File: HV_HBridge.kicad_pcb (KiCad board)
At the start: 2 copper layers, 1 part

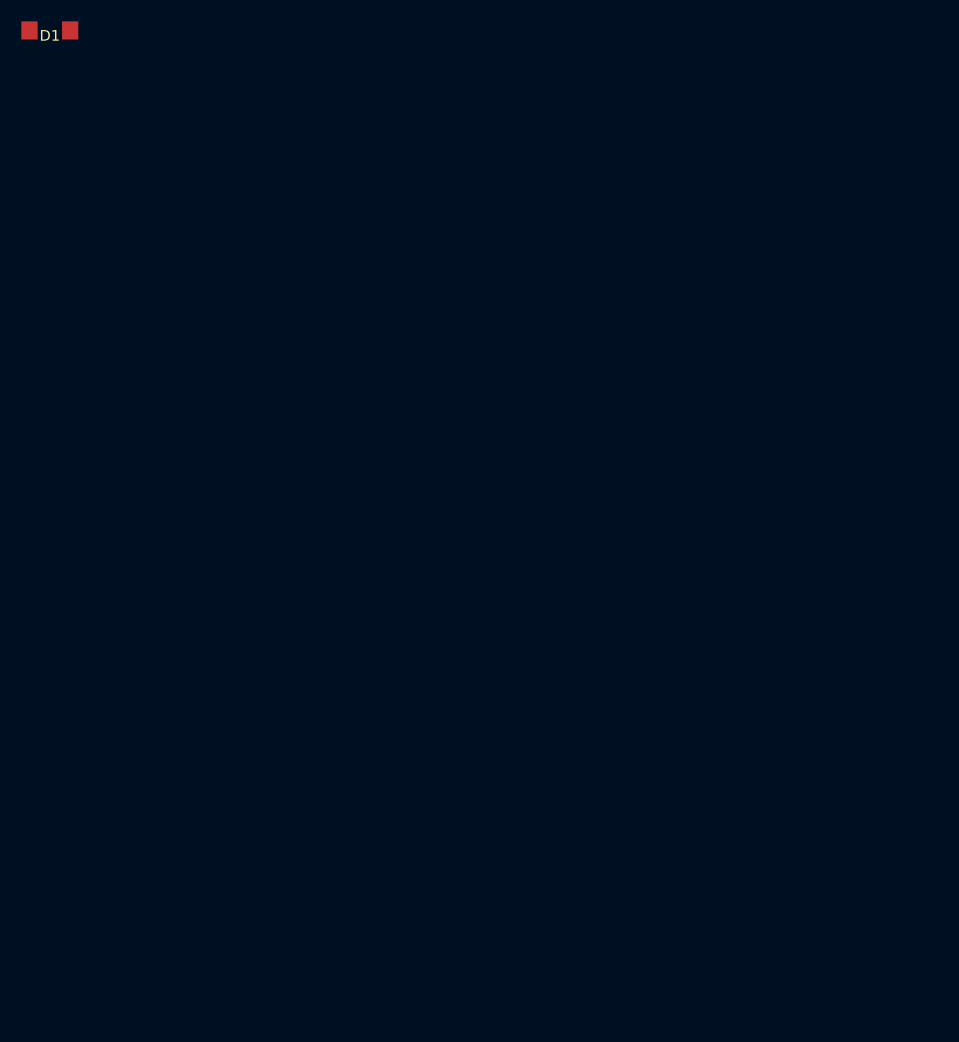
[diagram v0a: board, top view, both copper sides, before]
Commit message: updated to latest version
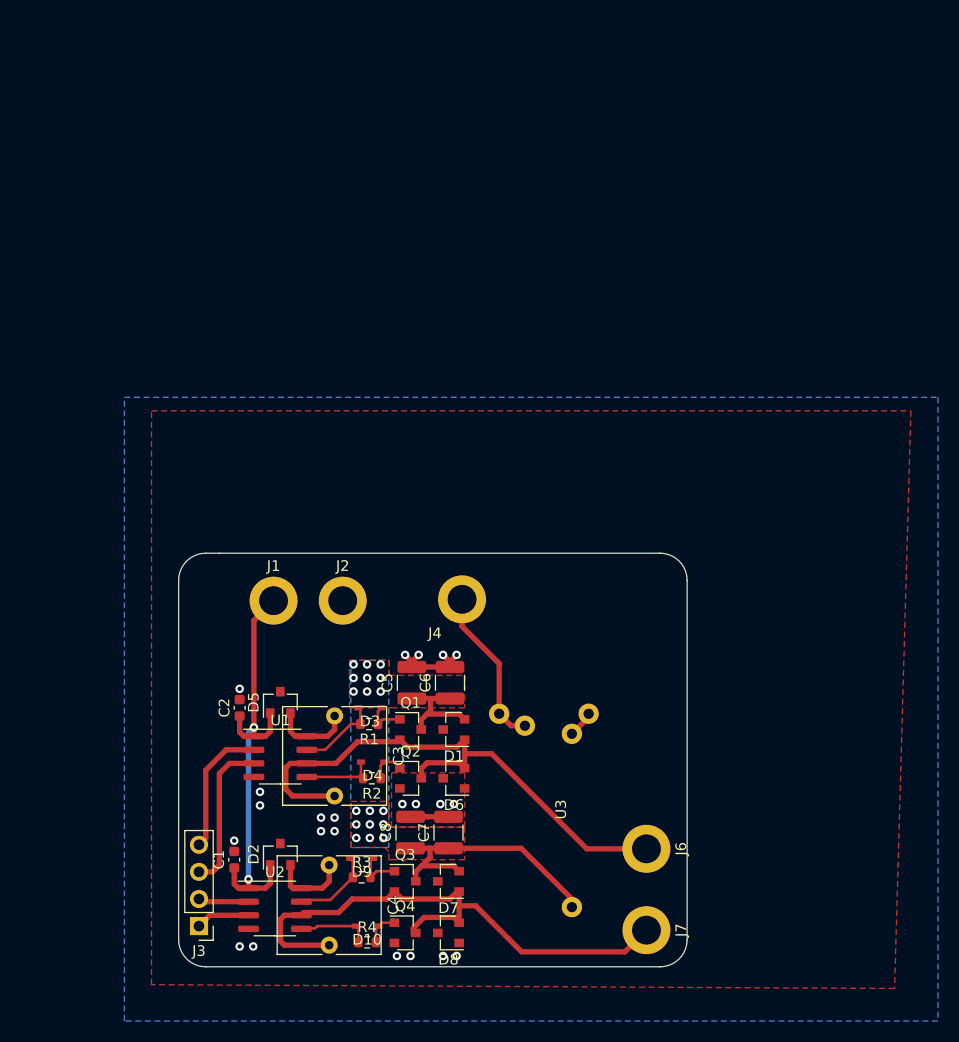
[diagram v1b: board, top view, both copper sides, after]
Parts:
- added C1: 100n 25V, Capacitor_SMD:C_0603_1608Metric, F.Cu at (106.8, 68.7)
- added C2: 100n 25V, Capacitor_SMD:C_0603_1608Metric, F.Cu at (107.3, 54.5)
- added C3: 1u 630V, Capacitor_THT:C_Rect_L9.0mm_W9.5mm_P7.50mm_MKT, F.Cu at (116.2, 55.2)
- added C4: 1u 630V, Capacitor_THT:C_Rect_L9.0mm_W9.5mm_P7.50mm_MKT, F.Cu at (115.7, 69.2)
- added C5: 100n 630V, Capacitor_SMD:C_1210_3225Metric, F.Cu at (123.4, 52.1)
- added C6: 100n 630V, Capacitor_SMD:C_1210_3225Metric, F.Cu at (127.0, 52.1)
- added C7: 100n 630V, Capacitor_SMD:C_1210_3225Metric, F.Cu at (126.9, 66.2)
- added C8: 100n 630V, Capacitor_SMD:C_1210_3225Metric, F.Cu at (123.3, 66.2)
- added D10: D, HBREMS_Hbridge:SOD-323, F.Cu at (119.3, 74.9)
- added D2: BAS101, Package_TO_SOT_SMD:SOT-23, F.Cu at (111.1, 68.2)
- added D3: D, HBREMS_Hbridge:SOD-323, F.Cu at (119.5, 54.5)
- added D4: D, HBREMS_Hbridge:SOD-323, F.Cu at (119.8, 59.6)
- added D5: BAS101, Package_TO_SOT_SMD:SOT-23, F.Cu at (111.1, 54.0)
- added D6: BAS101, Package_TO_SOT_SMD:SOT-23, F.Cu at (127.4, 61.1)
- added D7: BAS101, Package_TO_SOT_SMD:SOT-23, F.Cu at (126.9, 70.7)
- added D8: BAS101, Package_TO_SOT_SMD:SOT-23, F.Cu at (126.9, 75.6)
- added D9: D, HBREMS_Hbridge:SOD-323, F.Cu at (118.7, 68.6)
- added J1: Conn_01x01_Male, MountingHole:MountingHole_2.7mm_M2.5_ISO7380_Pad, F.Cu at (110.5, 44.5)
- added J2: Conn_01x01_Male, MountingHole:MountingHole_2.7mm_M2.5_ISO7380_Pad, F.Cu at (117.0, 44.5)
- added J3: Conn_01x04, Connector_PinHeader_2.54mm:PinHeader_1x04_P2.54mm_Vertical, F.Cu at (103.5, 74.9)
- added J4: Conn_01x01_Male, MountingHole:MountingHole_2.7mm_M2.5_ISO7380_Pad, F.Cu at (128.1, 44.3)
- added J6: Conn_01x01_Male, MountingHole:MountingHole_2.7mm_M2.5_ISO7380_Pad, F.Cu at (145.4, 67.7)
- added J7: Conn_01x01_Male, MountingHole:MountingHole_2.7mm_M2.5_ISO7380_Pad, F.Cu at (145.4, 75.3)
- added Q1: BSS127, Package_TO_SOT_SMD:SOT-23, F.Cu at (123.3, 56.5)
- added Q2: BSS127, Package_TO_SOT_SMD:SOT-23, F.Cu at (123.3, 61.1)
- added Q3: BSS127, Package_TO_SOT_SMD:SOT-23, F.Cu at (122.8, 70.7)
- added Q4: BSS127, Package_TO_SOT_SMD:SOT-23, F.Cu at (122.8, 75.6)
- added R1: 27R 50V, Resistor_SMD:R_0603_1608Metric, F.Cu at (119.4, 56.0)
- added R2: 27R 50V, Resistor_SMD:R_0603_1608Metric, F.Cu at (119.7, 61.1)
- added R3: 27R 50V, Resistor_SMD:R_0603_1608Metric, F.Cu at (118.7, 70.4)
- added R4: 27R 50V, Resistor_SMD:R_0603_1608Metric, F.Cu at (119.3, 76.5)
- added U1: IR2104, Package_SO:SOIC-8_3.9x4.9mm_P1.27mm, F.Cu at (111.1, 59.1)
- added U2: IR2104, Package_SO:SOIC-8_3.9x4.9mm_P1.27mm, F.Cu at (110.6, 73.3)
- added U3: A03P-12, HBREMS_Hbridge:A03P-12, F.Cu at (135.9, 63.5)
- D1: value D_Schottky_Small -> BAS101; footprint HV_HBridge:FM2500 -> Package_TO_SOT_SMD:SOT-23
- moved D1 75.6 mm to (127.4, 56.5), turned to 180 degrees
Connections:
- D1 pad 1: Net-(C1-Pad1) -> /hbridge1/LOAD1
- D1 pad 2: VDD -> VCC
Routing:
- net /hbridge1/LOAD1: track 0.00 -> 54.0 mm
- net /hbridge1/LOAD2: track 0.00 -> 53.9 mm
- net VDD: track 0.00 -> 42.1 mm, vias 0 -> 2
- net VCC: track 0.00 -> 35.8 mm, vias 0 -> 18
- net V_Var: track 0.00 -> 15.0 mm
- net GND: track 0.00 -> 14.7 mm, vias 0 -> 22
- net /hbridge1/PWM1_EN: track 0.00 -> 14.4 mm
- net /hbridge1/PWM1: track 0.00 -> 12.5 mm
- net HS_A: track 0.00 -> 7.62 mm
- net HS_B: track 0.00 -> 7.59 mm
- net Net-(C3-Pad1): track 0.00 -> 7.58 mm
- net Net-(C4-Pad1): track 0.00 -> 7.47 mm
- net LS_A: track 0.00 -> 6.93 mm
- net LS_B: track 0.00 -> 6.81 mm
- net /hbridge1/PWM2_EN: track 0.00 -> 5.63 mm
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- added copper zone on B.Cu, net GND
- added copper zone on F.Cu, net GND
- added copper zone on B.Cu, net VCC
- added copper zone on F.Cu, net VCC
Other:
- board outline added: 47.6 x 38.7 mm
- net class HV added: clearance 0.8, trace_width 0.25, via_dia 0.8, via_drill 0.4
- board text added: "LOAD1"
- board text added: "LOAD2"
- board text added: "L_GND"
- board text added: "L_VDD"
- board text added: "Tobias Gent HBREMS_HBridge"
- board text added: "V_CTRL"

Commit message: changed board fsilk to 'HV_HBridge'
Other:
- board text added: "Tobias Gent HV_HBridge"
- board text removed: "Tobias Gent HBREMS_HBridge"
